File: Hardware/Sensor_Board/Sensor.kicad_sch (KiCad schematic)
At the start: 16 parts, among them U301 ICE40UL1K-CM36AI, U401 BNO086, Y401 32.768 kHz

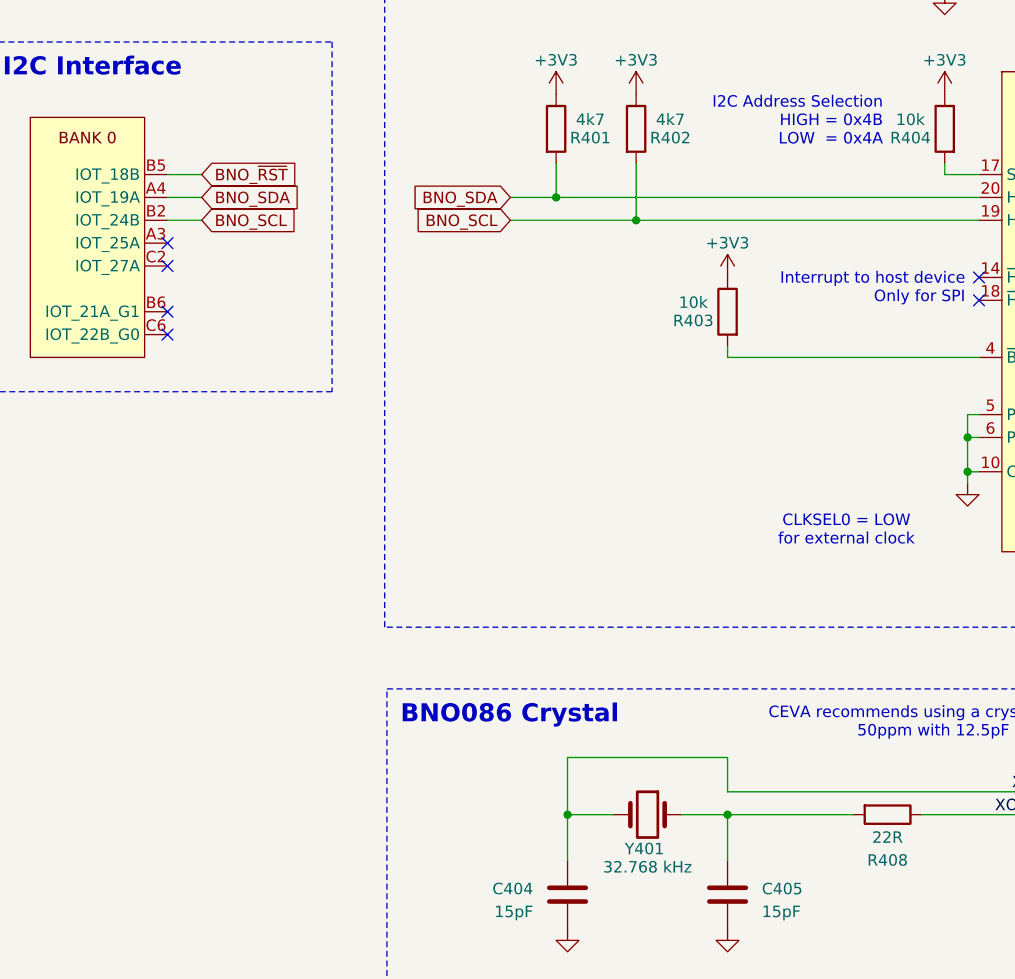
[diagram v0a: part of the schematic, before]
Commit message: Pushing before updating KiCad
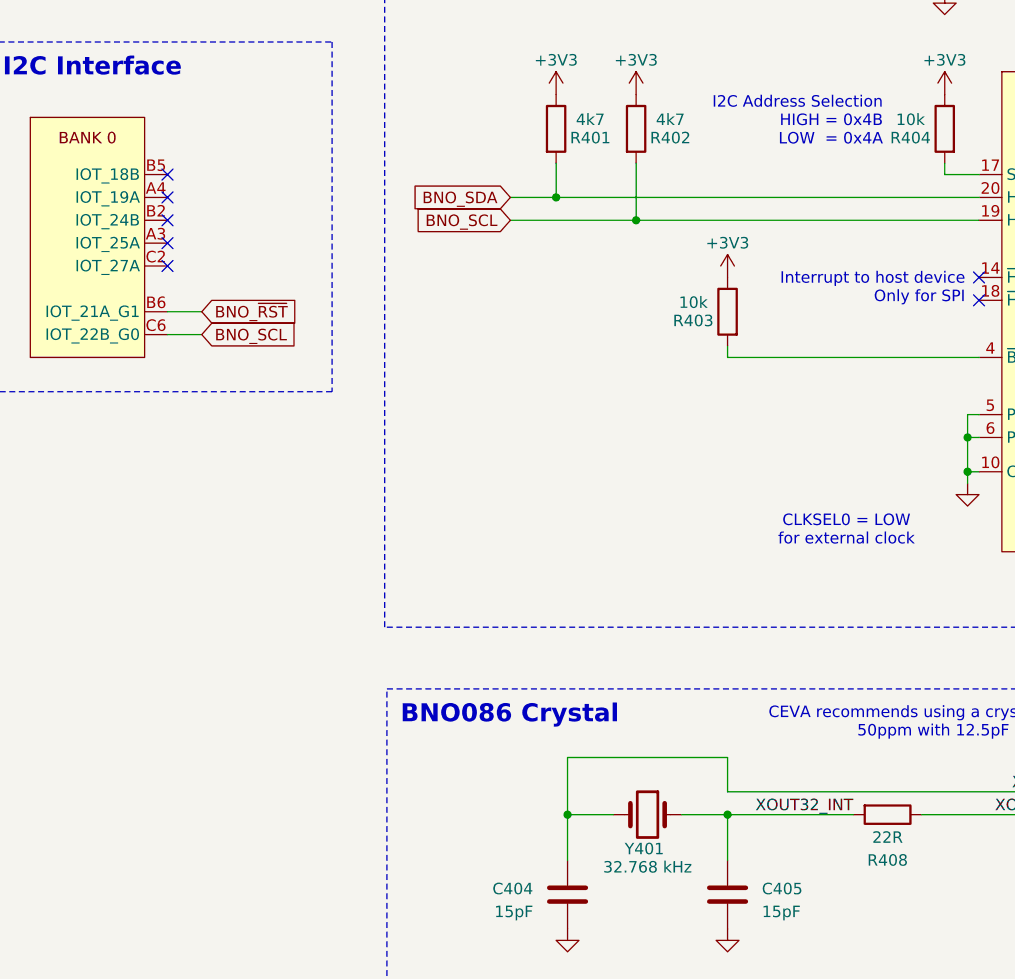
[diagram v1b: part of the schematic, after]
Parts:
- R401, R402, R403, R404, R405, R406, R407: footprint (none) -> Resistor_SMD:R_0402_1005Metric
- U301: footprint Package_BGA:UCBGA-36_2.5x2.5mm_Layout6x6_P0.4mm -> Custom_VoxLink_Footprints:ICE40UL1K_UCBGA-36
- U401: footprint (none) -> Package_LGA:LGA-28_5.2x3.8mm_P0.5mm
- Y401: footprint (none) -> Crystal:Crystal_SMD_MicroCrystal_CC8V-T1A-2Pin_2.0x1.2mm
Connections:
- net BNO_SCL: now also U301.C6 (IOT_22B_G0); no longer U301.B2 (IOT_24B)
- net BNO_SDA: no longer U301.A4 (IOT_19A)
- net BNO_~{RST}: now also U301.B6 (IOT_21A_G1); no longer U301.B5 (IOT_18B)
- net XOUT32_INT: now reaches C405.1, R408.2, Y401.1
- no-connect marks 6 -> 7
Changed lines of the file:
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@@
 	)
 	(no_connect
+		(at 144.78 102.87)
+	)
+	(no_connect
 		(at 54.61 96.52)
 	)
 	(no_connect
-		(at 54.61 106.68)
+		(at 54.61 99.06)
 	)
 	(no_connect
-		(at 144.78 102.87)
+		(at 144.78 100.33)
 	)
 	(no_connect
-		(at 54.61 99.06)
+		(at 54.61 93.98)
 	)
 	(no_connect
-		(at 54.61 104.14)
+		(at 54.61 88.9)
 	)
 	(no_connect
-		(at 144.78 100.33)
+		(at 54.61 91.44)
 	)
 	(wire
@@
 	(wire
 		(pts
-			(xy 54.61 88.9) (xy 58.42 88.9)
+			(xy 54.61 106.68) (xy 58.42 106.68)
 		)
 		(stroke
@@
 	(wire
 		(pts
-			(xy 54.61 93.98) (xy 58.42 93.98)
-		)
-		(stroke
-			(width 0)
-			(type default)
-		)
-	)
-	(wire
-		(pts
-			(xy 54.61 91.44) (xy 58.42 91.44)
+			(xy 54.61 104.14) (xy 58.42 104.14)
 		)
 		(stroke
@@
 		)
 	)
+	(label "XOUT32_INT"
+		(at 130.81 160.02 180)
+		(effects
+			(font
+				(size 1.27 1.27)
+			)
+			(justify right bottom)
+		)
+	)
 	(label "XIN32"
 		(at 189.23 113.03 180)
@@
 	(global_label "BNO_SCL"
 		(shape input)
-		(at 58.42 93.98 0)
+		(at 58.42 106.68 0)
 		(fields_autoplaced yes)
 		(effects
@@
 		)
 		(property "Intersheetrefs" "${INTERSHEET_REFS}"
-			(at 69.8114 93.98 0)
+			(at 69.8114 106.68 0)
 			(effects
 				(font
@@
 		)
 	)
-	(global_label "BNO_SDA"
-		(shape input)
-		(at 58.42 91.44 0)
-		(fields_autoplaced yes)
-		(effects
-			(font
-				(size 1.27 1.27)
-			)
-			(justify left)
-		)
-		(property "Intersheetrefs" "${INTERSHEET_REFS}"
-			(at 69.8719 91.44 0)
-			(effects
-				(font
-					(size 1.27 1.27)
-				)
-				(justify left)
-				(hide yes)
-			)
-		)
-	)
 	(global_label "BNO_~{RST}"
 		(shape input)
-		(at 58.42 88.9 0)
+		(at 58.42 104.14 0)
 		(fields_autoplaced yes)
 		(effects
@@
 		)
 		(property "Intersheetrefs" "${INTERSHEET_REFS}"
-			(at 69.7509 88.9 0)
+			(at 69.7509 104.14 0)
 			(effects
 				(font
@@
 			)
 		)
-		(property "Datasheet" "https://eu.mouser.com/ProductDetail/81-GCM1555G1H100JA6D"
+		(property "Datasheet" "https://www.mouser.sk/ProductDetail/Murata-Electronics/GRM1555C1H150FA01D?qs=ouTquLLW2S7neucAALMxaw%3D%3D"
 			(at 99.06 168.91 0)
 			(effects
@@
 			)
 		)
-		(property "Footprint" ""
+		(property "Footprint" "Package_LGA:LGA-28_5.2x3.8mm_P0.5mm"
 			(at 147.32 91.44 0)
 			(effects
@@
 			)
 		)
-		(property "Footprint" ""
+		(property "Footprint" "Resistor_SMD:R_0402_1005Metric"
 			(at 142.748 83.82 90)
 			(effects
@@
 			)
 		)
-		(property "Datasheet" ""
+		(property "Datasheet" "https://www.mouser.sk/ProductDetail/Vishay/CRCW040210K0JNED?qs=sGAEpiMZZMtlubZbdhIBIFsfWmIKznfcMCgOmcXe42g%3D"
 			(at 140.97 83.82 0)
 			(effects
@@
 			)
 		)
-		(property "Footprint" ""
+		(property "Footprint" "Resistor_SMD:R_0402_1005Metric"
 			(at 118.618 104.14 90)
 			(effects
@@
 			)
 		)
-		(property "Datasheet" ""
+		(property "Datasheet" "https://www.mouser.sk/ProductDetail/Vishay/CRCW040210K0JNED?qs=sGAEpiMZZMtlubZbdhIBIFsfWmIKznfcMCgOmcXe42g%3D"
 			(at 116.84 104.14 0)
 			(effects
@@
 			)
 		)
-		(property "Footprint" ""
+		(property "Footprint" "Resistor_SMD:R_0402_1005Metric"
 			(at 96.012 83.82 90)
 			(effects
@@
 			)
 		)
-		(property "Datasheet" ""
+		(property "Datasheet" "https://www.mouser.sk/ProductDetail/Vishay/CRCW04024K70JNED?qs=sGAEpiMZZMtlubZbdhIBIPcJW8E8ShybHI4602K%2FbXw%3D"
 			(at 97.79 83.82 0)
 			(effects
@@
 			)
 		)
-		(property "Footprint" "Package_BGA:UCBGA-36_2.5x2.5mm_Layout6x6_P0.4mm"
+		(property "Footprint" "Custom_VoxLink_Footprints:ICE40UL1K_UCBGA-36"
 			(at 45.72 95.25 0)
 			(effects
@@
 			)
 		)
-		(property "Footprint" ""
+		(property "Footprint" "Crystal:Crystal_SMD_MicroCrystal_CC8V-T1A-2Pin_2.0x1.2mm"
 			(at 107.95 160.02 0)
 			(effects
@@
 			)
 		)
-		(property "Footprint" ""
+		(property "Footprint" "Resistor_SMD:R_0402_1005Metric"
 			(at 104.902 83.82 90)
 			(effects
@@
 			)
 		)
-		(property "Datasheet" ""
+		(property "Datasheet" "https://www.mouser.sk/ProductDetail/Vishay/CRCW04024K70JNED?qs=sGAEpiMZZMtlubZbdhIBIPcJW8E8ShybHI4602K%2FbXw%3D"
 			(at 106.68 83.82 0)
 			(effects
@@
 			)
 		)
-		(property "Footprint" ""
+		(property "Footprint" "Resistor_SMD:R_0402_1005Metric"
 			(at 202.692 92.71 90)
 			(effects
@@
 			)
 		)
-		(property "Datasheet" ""
+		(property "Datasheet" "https://www.mouser.sk/ProductDetail/Vishay/CRCW04024K70JNED?qs=sGAEpiMZZMtlubZbdhIBIPcJW8E8ShybHI4602K%2FbXw%3D"
 			(at 204.47 92.71 0)
 			(effects
@@
 			)
 		)
-		(property "Footprint" ""
+		(property "Footprint" "Resistor_SMD:R_0402_1005Metric"
 			(at 211.582 92.71 90)
 			(effects
@@
 			)
 		)
-		(property "Datasheet" ""
+		(property "Datasheet" "https://www.mouser.sk/ProductDetail/Vishay/CRCW04024K70JNED?qs=sGAEpiMZZMtlubZbdhIBIPcJW8E8ShybHI4602K%2FbXw%3D"
 			(at 213.36 92.71 0)
 			(effects
@@
 			)
 		)
-		(property "Datasheet" ""
+		(property "Datasheet" "https://www.mouser.sk/ProductDetail/Murata-Electronics/GCM155R71H104KE02J?qs=hNud%2FORuBR1wlwGPFWBVDg%3D%3D"
 			(at 152.4 64.77 0)
 			(effects
@@
 			)
 		)
-		(property "Datasheet" "https://eu.mouser.com/ProductDetail/81-GCM1555G1H100JA6D"
+		(property "Datasheet" "https://www.mouser.sk/ProductDetail/Murata-Electronics/GCM155R71H104KE02J?qs=hNud%2FORuBR1wlwGPFWBVDg%3D%3D"
 			(at 181.61 128.27 0)
 			(effects
@@
 			)
 		)
-		(property "Datasheet" "https://eu.mouser.com/ProductDetail/81-GCM1555G1H100JA6D"
+		(property "Datasheet" "https://www.mouser.sk/ProductDetail/Murata-Electronics/GRM1555C1H150FA01D?qs=ouTquLLW2S7neucAALMxaw%3D%3D"
 			(at 116.84 168.91 0)
 			(effects
@@
 			)
 		)
-		(property "Footprint" ""
+		(property "Footprint" "Resistor_SMD:R_0402_1005Metric"
 			(at 181.102 83.82 90)
 			(effects
@@
 			)
 		)
-		(property "Datasheet" ""
+		(property "Datasheet" "https://www.mouser.sk/ProductDetail/Vishay/CRCW040210K0JNED?qs=sGAEpiMZZMtlubZbdhIBIFsfWmIKznfcMCgOmcXe42g%3D"
 			(at 182.88 83.82 0)
 			(effects
@@
 			)
 		)
-		(property "Datasheet" ""
+		(property "Datasheet" "https://www.mouser.sk/ProductDetail/Murata-Electronics/GCM155R71H104KE02J?qs=hNud%2FORuBR1wlwGPFWBVDg%3D%3D"
 			(at 140.97 64.77 0)
 			(effects
